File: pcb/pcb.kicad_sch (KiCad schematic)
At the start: 16 parts, among them CN1 1x4, CN10 1x2, CN11 1x2, CN2 1x8, CN3 1x8, CN4 1x8, CN5 1x4, CN6 1x2, CN7 1x2, SW1 switch_3x4, SW2 switch_3x4, SW3 219-3LPST

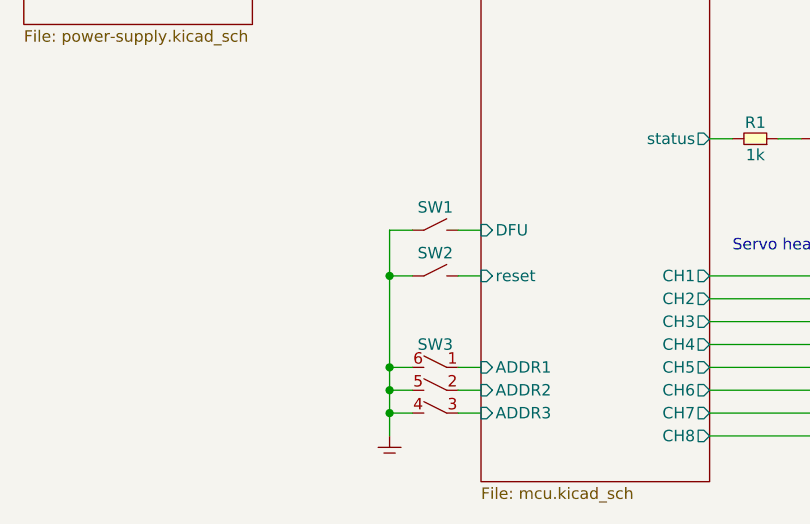
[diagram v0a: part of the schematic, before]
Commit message: worked on pinout
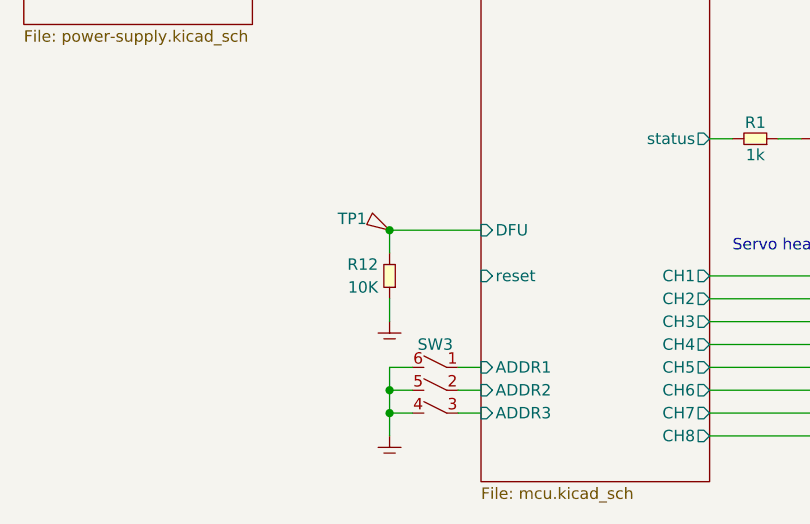
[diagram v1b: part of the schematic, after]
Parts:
- removed SW1, SW2: switch_3x4, buttons:sw_3x4, symbol switches:switch_3x4
- added R12: 10K, SMT:0603, symbol generic:R
- added TP1: test_point, PCB:test_point, symbol PCB:test_point
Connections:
- net GND: now also R12.1
- net MCU/DFU: now also R12.2, TP1.1 (TP)
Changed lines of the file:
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@@
     (comment 1 "User interfaces")
   )
-  (junction (at 129.54 121.92) (diameter 0) (color 0 0 0 0)
-  )
   (junction (at 251.46 109.22) (diameter 0) (color 0 0 0 0)
   )
@@
   (junction (at 203.2 132.08) (diameter 0) (color 0 0 0 0)
   )
+  (junction (at 129.54 116.84) (diameter 0) (color 0 0 0 0)
+  )
   (junction (at 129.54 137.16) (diameter 0) (color 0 0 0 0)
   )
   (junction (at 203.2 129.54) (diameter 0) (color 0 0 0 0)
   )
-  (junction (at 129.54 132.08) (diameter 0) (color 0 0 0 0)
-  )
   (junction (at 190.5 124.46) (diameter 0) (color 0 0 0 0)
   )
@@
     (stroke (width 0) (type default))
   )
-  (wire (pts (xy 129.54 116.84) (xy 132.08 116.84))
-    (stroke (width 0) (type default))
-  )
-  (wire (pts (xy 129.54 132.08) (xy 129.54 121.92))
-    (stroke (width 0) (type default))
-  )
   (wire (pts (xy 203.2 137.16) (xy 205.74 137.16))
     (stroke (width 0) (type default))
   )
+  (wire (pts (xy 129.54 116.84) (xy 129.54 119.38))
+    (stroke (width 0) (type default))
+  )
   (wire (pts (xy 203.2 127) (xy 205.74 127))
     (stroke (width 0) (type default))
@@
     (stroke (width 0) (type default))
   )
-  (wire (pts (xy 137.16 116.84) (xy 139.7 116.84))
-    (stroke (width 0) (type default))
-  )
   (wire (pts (xy 137.16 132.08) (xy 139.7 132.08))
     (stroke (width 0) (type default))
@@
     (stroke (width 0) (type default))
   )
+  (wire (pts (xy 139.7 116.84) (xy 129.54 116.84))
+    (stroke (width 0) (type default))
+  )
   (wire (pts (xy 231.14 99.06) (xy 228.6 99.06))
     (stroke (width 0) (type default))
@@
     (stroke (width 0) (type default))
   )
-  (wire (pts (xy 129.54 121.92) (xy 132.08 121.92))
-    (stroke (width 0) (type default))
-  )
   (wire (pts (xy 203.2 127) (xy 203.2 124.46))
     (stroke (width 0) (type default))
   )
-  (wire (pts (xy 137.16 121.92) (xy 139.7 121.92))
-    (stroke (width 0) (type default))
-  )
   (wire (pts (xy 193.04 114.3) (xy 190.5 114.3))
     (stroke (width 0) (type default))
@@
     (stroke (width 0) (type default))
   )
+  (wire (pts (xy 129.54 124.46) (xy 129.54 127))
+    (stroke (width 0) (type default))
+  )
   (wire (pts (xy 233.68 83.82) (xy 233.68 88.9))
     (stroke (width 0) (type default))
@@
   )
   (wire (pts (xy 256.54 88.9) (xy 261.62 88.9))
-    (stroke (width 0) (type default))
-  )
-  (wire (pts (xy 129.54 121.92) (xy 129.54 116.84))
     (stroke (width 0) (type default))
   )
@@
     )
   )
-  (symbol (lib_id "switches:switch_3x4") (at 134.62 116.84 0) (unit 1)
+  (symbol (lib_id "generic:GND") (at 129.54 127 0) (unit 1)
     (in_bom yes) (on_board yes) (dnp no) (fields_autoplaced)
-    (property "Reference" "SW1" (at 134.62 114.3 0)
-      (effects (font (size 1.27 1.27)))
-    )
-    (property "Value" "switch_3x4" (at 134.62 114.3 0)
-      (effects (font (size 1.27 1.27)) hide)
-    )
-    (property "Footprint" "buttons:sw_3x4" (at 134.62 118.11 0)
-      (effects (font (size 1.27 1.27)) hide)
-    )
-    (property "Datasheet" "" (at 134.62 116.84 0)
-      (effects (font (size 1.27 1.27)) hide)
-    )
-    (pin "1")
-    (pin "2")
-    (pin "3")
-    (pin "4")
-    (instances
-      (project "pcb"
-        (path "/6bb3bad6-1a89-4624-b34d-6ddda7dd16d2"
-          (reference "SW1") (unit 1)
+    (property "Reference" "#GND02" (at 133.35 125.73 0)
+      (effects (font (size 1.27 1.27)) hide)
+    )
+    (property "Value" "GND" (at 133.35 127 0)
+      (effects (font (size 1.27 1.27)) hide)
+    )
+    (property "Footprint" "" (at 129.54 127 0)
+      (effects (font (size 1.27 1.27)) hide)
+    )
+    (property "Datasheet" "" (at 129.54 127 0)
+      (effects (font (size 1.27 1.27)) hide)
+    )
+    (pin "~")
+    (instances
+      (project "pcb"
+        (path "/6bb3bad6-1a89-4624-b34d-6ddda7dd16d2"
+          (reference "#GND02") (unit 1)
         )
       )
@@
     )
   )
-  (symbol (lib_id "switches:switch_3x4") (at 134.62 121.92 0) (unit 1)
-    (in_bom yes) (on_board yes) (dnp no)
-    (property "Reference" "SW2" (at 134.62 119.38 0)
-      (effects (font (size 1.27 1.27)))
-    )
-    (property "Value" "switch_3x4" (at 134.62 119.38 0)
-      (effects (font (size 1.27 1.27)) hide)
-    )
-    (property "Footprint" "buttons:sw_3x4" (at 134.62 123.19 0)
-      (effects (font (size 1.27 1.27)) hide)
-    )
-    (property "Datasheet" "" (at 134.62 121.92 0)
-      (effects (font (size 1.27 1.27)) hide)
-    )
-    (pin "1")
-    (pin "2")
-    (pin "3")
-    (pin "4")
-    (instances
-      (project "pcb"
-        (path "/6bb3bad6-1a89-4624-b34d-6ddda7dd16d2/19469851-aeaf-466c-9786-c0d0ae531cf4"
-          (reference "SW2") (unit 1)
-        )
-        (path "/6bb3bad6-1a89-4624-b34d-6ddda7dd16d2"
-          (reference "SW2") (unit 1)
-        )
-      )
-    )
-  )
   (symbol (lib_id "generic:GND") (at 129.54 139.7 0) (unit 1)
     (in_bom yes) (on_board yes) (dnp no) (fields_autoplaced)
@@
     )
   )
+  (symbol (lib_id "PCB:test_point") (at 129.54 116.84 0) (mirror y) (unit 1)
+    (in_bom yes) (on_board yes) (dnp no)
+    (property "Reference" "TP1" (at 127 115.57 0)
+      (effects (font (size 1.27 1.27)) (justify left))
+    )
+    (property "Value" "test_point" (at 129.54 114.3 0)
+      (effects (font (size 1.27 1.27)) hide)
+    )
+    (property "Footprint" "PCB:test_point" (at 127 118.11 0)
+      (effects (font (size 1.27 1.27)) hide)
+    )
+    (property "Datasheet" "" (at 129.54 116.84 0)
+      (effects (font (size 1.27 1.27)) hide)
+    )
+    (pin "1")
+    (instances
+      (project "pcb"
+        (path "/6bb3bad6-1a89-4624-b34d-6ddda7dd16d2"
+          (reference "TP1") (unit 1)
+        )
+      )
+    )
+  )
   (symbol (lib_id "pin_headers:1x2") (at 60.96 78.74 0) (mirror y) (unit 1)
     (in_bom yes) (on_board yes) (dnp no) (fields_autoplaced)
@@
         )
       )
+    )
+  )
+  (symbol (lib_name "R_1") (lib_id "generic:R") (at 129.54 121.92 270) (mirror x) (unit 1)
+    (in_bom yes) (on_board yes) (dnp no)
+    (property "Reference" "R12" (at 128.27 120.65 90)
+      (effects (font (size 1.27 1.27)) (justify right))
+    )
+    (property "Value" "10K" (at 128.27 123.19 90)
+      (effects (font (size 1.27 1.27)) (justify right))
+    )
+    (property "Footprint" "SMT:0603" (at 128.905 124.46 0)
+      (effects (font (size 1.27 1.27)) hide)
+    )
+    (property "Datasheet" "" (at 129.54 121.92 0)
+      (effects (font (size 1.27 1.27)) hide)
+    )
+    (pin "1")
+    (pin "2")
+    (instances
+      (project "pcb"
+        (path "/6bb3bad6-1a89-4624-b34d-6ddda7dd16d2"
+          (reference "R12") (unit 1)
+        )
+      )
